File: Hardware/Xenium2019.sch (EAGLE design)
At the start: 20 parts, among them J1 SM10B-SRSS-TB, Q1 310mA/60V/1.6Ω, Q2 310mA/60V/1.6Ω, Q3 310mA/60V/1.6Ω, Q4 310mA/60V/1.6Ω, U1 XC9572XL-10VQG64, U2 AM29LV160M

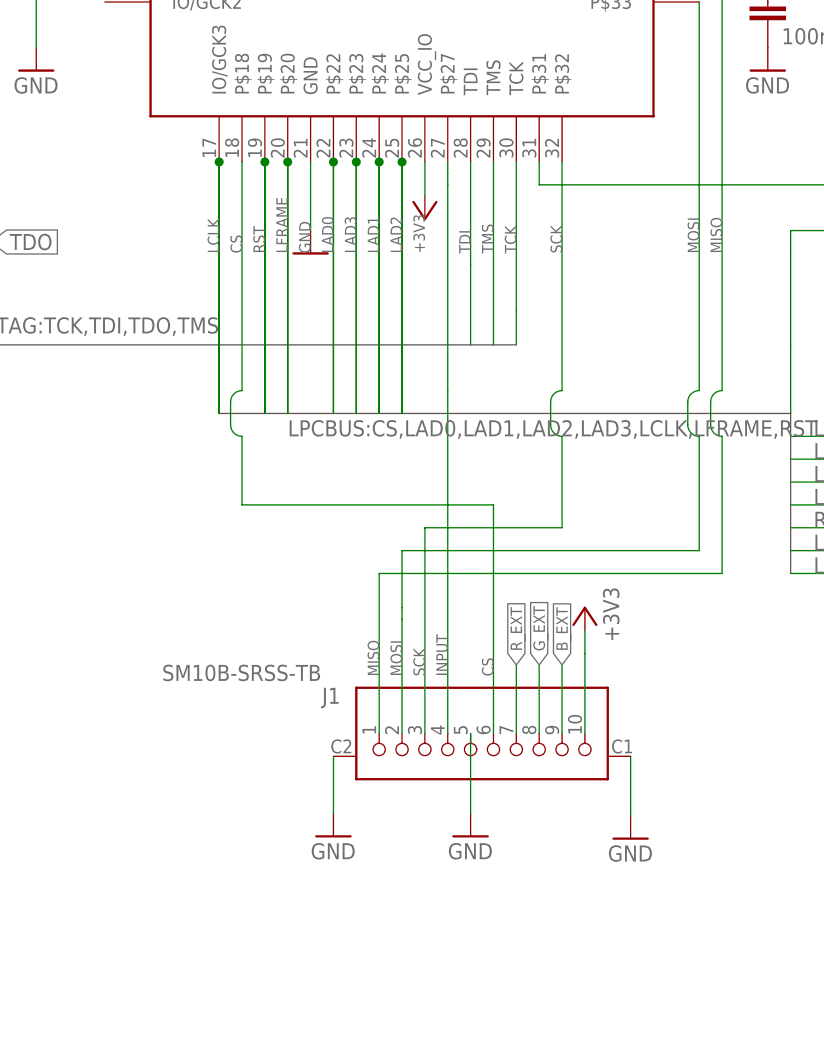
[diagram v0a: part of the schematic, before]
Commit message: Update: added pads
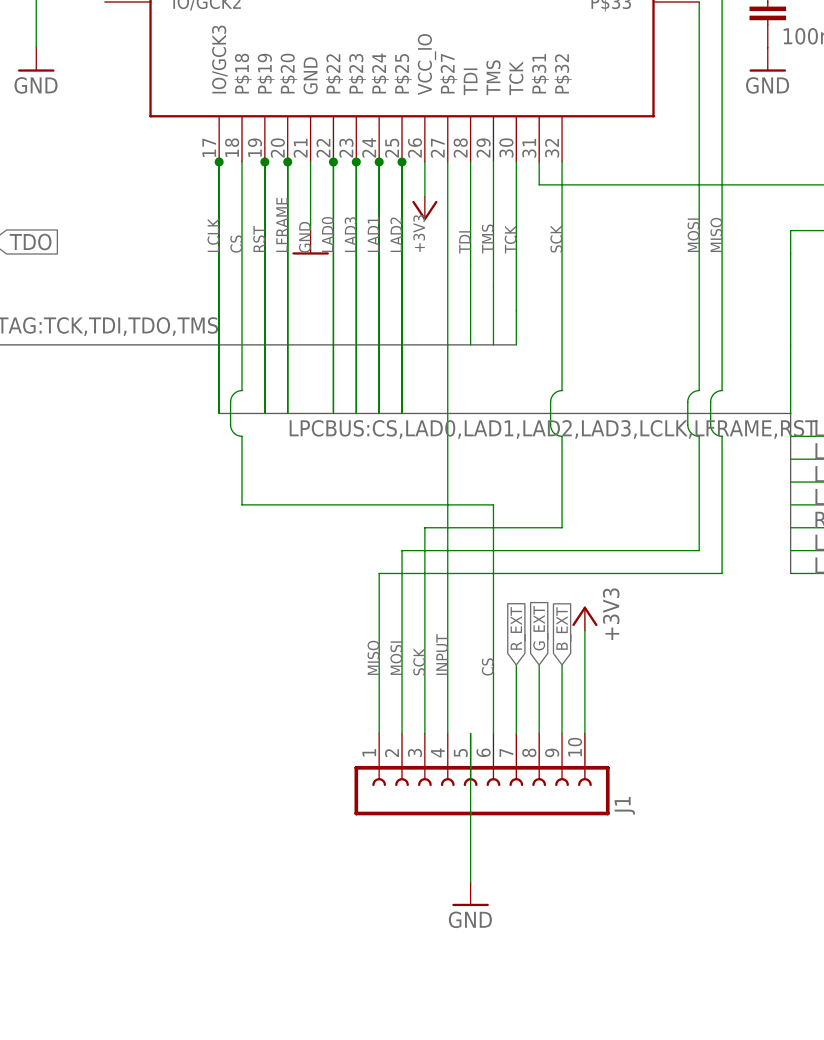
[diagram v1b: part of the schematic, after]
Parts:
- J1: value SM10B-SRSS-TB -> (none); device my-library:SM10B-SRSS-TB -> con-lsta:FE10-1
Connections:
- net GND: no longer J1.MNT1, J1.MNT2
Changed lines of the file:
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@@
 <?xml version="1.0" encoding="utf-8"?>
 <!DOCTYPE eagle SYSTEM "eagle.dtd">
-<eagle version="9.5.1">
+<eagle version="9.6.2">
 <drawing>
 <settings>
@@
 <part name="Q4" library="zetex" library_urn="urn:adsk.eagle:library:418" deviceset="NMOSSOT23" device="" package3d_urn="urn:adsk.eagle:package:30981/1" override_package3d_urn="urn:adsk.eagle:package:13055076/2" override_package_urn="urn:adsk.eagle:footprint:30948/1" value="310mA/60V/1.6Ω"/>
 <part name="Q3" library="zetex" library_urn="urn:adsk.eagle:library:418" deviceset="NMOSSOT23" device="" package3d_urn="urn:adsk.eagle:package:30981/1" override_package3d_urn="urn:adsk.eagle:package:13055076/2" override_package_urn="urn:adsk.eagle:footprint:30948/1" value="310mA/60V/1.6Ω"/>
-<part name="J1" library="my-library" library_urn="urn:adsk.eagle:library:7078210" deviceset="SM10B-SRSS-TB" device="" override_package3d_urn="urn:adsk.eagle:package:13505000/4" override_package_urn="urn:adsk.eagle:footprint:13505001/2"/>
-<part name="GND10" library="supply1" library_urn="urn:adsk.eagle:library:371" deviceset="GND" device=""/>
-<part name="GND15" library="supply1" library_urn="urn:adsk.eagle:library:371" deviceset="GND" device=""/>
 <part name="FRAME1" library="frames" library_urn="urn:adsk.eagle:library:229" deviceset="A3L-LOC" device="" value="www"/>
 <part name="LPC" library="pinhead" library_urn="urn:adsk.eagle:library:325" deviceset="PINHD-2X7" device="" package3d_urn="urn:adsk.eagle:package:22478/2"/>
 <part name="TP1" library="testpad" library_urn="urn:adsk.eagle:library:385" deviceset="TP" device="TP13SQ" package3d_urn="urn:adsk.eagle:package:27974/1"/>
+<part name="J1" library="con-lsta" library_urn="urn:adsk.eagle:library:161" deviceset="FE10-1" device="" package3d_urn="urn:adsk.eagle:package:8192/1"/>
 </parts>
 <sheets>
@@
 <attribute name="VALUE" x="85.09" y="-35.56" size="1.778" layer="96" rot="R90"/>
 </instance>
-<instance part="GND6" gate="1" x="68.58" y="-57.15" smashed="yes">
-<attribute name="VALUE" x="66.04" y="-59.69" size="1.778" layer="96"/>
+<instance part="GND6" gate="1" x="68.58" y="-64.77" smashed="yes">
+<attribute name="VALUE" x="66.04" y="-67.31" size="1.778" layer="96"/>
 </instance>
 <instance part="GND7" gate="1" x="11.43" y="-17.78" smashed="yes">
@@
 <attribute name="NAME" x="-31.75" y="53.34" size="1.778" layer="95" font="vector" rot="MR0"/>
 </instance>
-<instance part="J1" gate="G$1" x="68.58" y="-43.18" smashed="yes" rot="MR270">
-<attribute name="NAME" x="52.07" y="-40.64" size="1.778" layer="95" rot="MR180"/>
-<attribute name="VALUE" x="34.29" y="-38.1" size="1.778" layer="96" rot="MR180"/>
-</instance>
-<instance part="GND10" gate="1" x="86.36" y="-57.404" smashed="yes">
-<attribute name="VALUE" x="83.82" y="-59.944" size="1.778" layer="96"/>
-</instance>
-<instance part="GND15" gate="1" x="53.34" y="-57.15" smashed="yes">
-<attribute name="VALUE" x="50.8" y="-59.69" size="1.778" layer="96"/>
-</instance>
 <instance part="FRAME1" gate="G$1" x="-121.92" y="-81.28" smashed="yes">
 <attribute name="SHEET" x="235.585" y="-76.2" size="2.54" layer="94" font="vector"/>
@@
 <instance part="TP1" gate="G$1" x="154.94" y="30.48" smashed="yes" rot="R270">
 <attribute name="TP_SIGNAL_NAME" x="153.67" y="29.21" size="1.778" layer="97" rot="R270"/>
+</instance>
+<instance part="J1" gate="G$1" x="68.58" y="-53.34" smashed="yes" rot="MR90">
+<attribute name="VALUE" x="53.34" y="-54.61" size="1.778" layer="96" rot="MR90"/>
+<attribute name="NAME" x="84.582" y="-54.61" size="1.778" layer="95" rot="MR90"/>
 </instance>
 </instances>
@@
 <net name="MOSI" class="0">
 <segment>
-<wire x1="60.96" y1="-33.02" x2="60.96" y2="-45.72" width="0.1524" layer="91"/>
+<wire x1="60.96" y1="-25.4" x2="60.96" y2="-45.72" width="0.1524" layer="91"/>
 <pinref part="U1" gate="G$1" pin="P$33"/>
 <wire x1="93.98" y1="35.56" x2="93.98" y2="-7.62" width="0.1524" layer="91"/>
 <wire x1="93.98" y1="-12.7" x2="93.98" y2="-25.4" width="0.1524" layer="91"/>
 <wire x1="93.98" y1="-25.4" x2="60.96" y2="-25.4" width="0.1524" layer="91"/>
-<wire x1="60.96" y1="-25.4" x2="60.96" y2="-31.75" width="0.1524" layer="91"/>
-<wire x1="60.96" y1="-31.75" x2="60.96" y2="-33.02" width="0.1524" layer="91"/>
 <label x="60.96" y="-39.37" size="1.27" layer="95" rot="R90"/>
-<pinref part="J1" gate="G$1" pin="2"/>
 <label x="93.98" y="7.62" size="1.27" layer="95" rot="R90"/>
 <wire x1="93.98" y1="-7.62" x2="92.71" y2="-8.89" width="0.1524" layer="91" curve="90"/>
 <wire x1="92.71" y1="-8.89" x2="92.71" y2="-11.43" width="0.1524" layer="91"/>
 <wire x1="92.71" y1="-11.43" x2="93.98" y2="-12.7" width="0.1524" layer="91" curve="90"/>
+<pinref part="J1" gate="G$1" pin="2"/>
 </segment>
 </net>
@@
 <segment>
 <pinref part="+3V6" gate="G$1" pin="+3V3"/>
-<wire x1="81.28" y1="-45.72" x2="81.28" y2="-36.83" width="0.1524" layer="91"/>
-<wire x1="81.28" y1="-36.83" x2="81.28" y2="-34.29" width="0.1524" layer="91"/>
+<wire x1="81.28" y1="-45.72" x2="81.28" y2="-34.29" width="0.1524" layer="91"/>
 <pinref part="J1" gate="G$1" pin="10"/>
 </segment>
@@
 <pinref part="U1" gate="G$1" pin="GND@2"/>
 <wire x1="50.8" y1="10.16" x2="50.8" y2="17.78" width="0.1524" layer="91"/>
-</segment>
-<segment>
-<wire x1="68.58" y1="-45.72" x2="68.58" y2="-54.61" width="0.1524" layer="91"/>
-<pinref part="GND6" gate="1" pin="GND"/>
-<pinref part="J1" gate="G$1" pin="5"/>
 </segment>
 <segment>
@@
 </segment>
 <segment>
-<pinref part="J1" gate="G$1" pin="MNT1"/>
-<pinref part="GND15" gate="1" pin="GND"/>
-<wire x1="53.34" y1="-48.26" x2="53.34" y2="-54.61" width="0.1524" layer="91"/>
-</segment>
-<segment>
-<pinref part="J1" gate="G$1" pin="MNT2"/>
-<pinref part="GND10" gate="1" pin="GND"/>
-<wire x1="86.36" y1="-48.26" x2="86.36" y2="-54.864" width="0.1524" layer="91"/>
+<pinref part="J1" gate="G$1" pin="5"/>
+<pinref part="GND6" gate="1" pin="GND"/>
+<wire x1="68.58" y1="-45.72" x2="68.58" y2="-62.23" width="0.1524" layer="91"/>
 </segment>
 </net>
@@
 <wire x1="43.18" y1="-20.32" x2="43.18" y2="-12.7" width="0.1524" layer="91"/>
 <label x="71.12" y="-39.37" size="1.27" layer="95" rot="R90"/>
-<pinref part="J1" gate="G$1" pin="6"/>
 <label x="43.18" y="7.62" size="1.27" layer="95" rot="R90"/>
 <wire x1="43.18" y1="-7.62" x2="43.18" y2="17.78" width="0.1524" layer="91"/>
@@
 <wire x1="41.91" y1="-8.89" x2="41.91" y2="-11.43" width="0.1524" layer="91"/>
 <wire x1="43.18" y1="-12.7" x2="41.91" y2="-11.43" width="0.1524" layer="91" curve="-90"/>
+<pinref part="J1" gate="G$1" pin="6"/>
 </segment>
 </net>
 <net name="INPUT" class="0">
 <segment>
-<wire x1="66.04" y1="-45.72" x2="66.04" y2="-7.62" width="0.1524" layer="91"/>
-<wire x1="66.04" y1="-7.62" x2="66.04" y2="15.24" width="0.1524" layer="91"/>
-<wire x1="66.04" y1="15.24" x2="66.04" y2="16.51" width="0.1524" layer="91"/>
+<wire x1="66.04" y1="-45.72" x2="66.04" y2="17.78" width="0.1524" layer="91"/>
 <pinref part="U1" gate="G$1" pin="P$27"/>
-<wire x1="66.04" y1="16.51" x2="66.04" y2="17.78" width="0.1524" layer="91"/>
+<label x="66.04" y="-39.37" size="1.27" layer="95" rot="R90"/>
 <pinref part="J1" gate="G$1" pin="4"/>
-<label x="66.04" y="-39.37" size="1.27" layer="95" rot="R90"/>
 </segment>
 </net>
@@
 <wire x1="78.74" y1="-22.86" x2="78.74" y2="-12.7" width="0.1524" layer="91"/>
 <label x="63.5" y="-39.37" size="1.27" layer="95" rot="R90"/>
-<pinref part="J1" gate="G$1" pin="3"/>
 <label x="78.74" y="7.62" size="1.27" layer="95" rot="R90"/>
 <wire x1="78.74" y1="-7.62" x2="78.74" y2="17.78" width="0.1524" layer="91"/>
@@
 <wire x1="77.47" y1="-8.89" x2="77.47" y2="-11.43" width="0.1524" layer="91"/>
 <wire x1="77.47" y1="-11.43" x2="78.74" y2="-12.7" width="0.1524" layer="91" curve="90"/>
+<pinref part="J1" gate="G$1" pin="3"/>
 </segment>
 </net>
@@
 <wire x1="96.52" y1="-27.94" x2="58.42" y2="-27.94" width="0.1524" layer="91"/>
 <wire x1="58.42" y1="-27.94" x2="58.42" y2="-45.72" width="0.1524" layer="91"/>
-<pinref part="J1" gate="G$1" pin="1"/>
 <label x="58.42" y="-39.37" size="1.27" layer="95" rot="R90"/>
 <label x="96.52" y="7.62" size="1.27" layer="95" rot="R90"/>
@@
 <wire x1="95.25" y1="-8.89" x2="95.25" y2="-11.43" width="0.1524" layer="91"/>
 <wire x1="95.25" y1="-11.43" x2="96.52" y2="-12.7" width="0.1524" layer="91" curve="90"/>
-</segment>
-</net>
+<pinref part="J1" gate="G$1" pin="1"/>
+</segment>
+</net>
